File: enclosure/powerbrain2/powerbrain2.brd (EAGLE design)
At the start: 24.8 x 64.8 mm, 45 parts, among them Q2 200mA/50V, Q3 200mA/50V, X2 ZX62D-B-5PA8

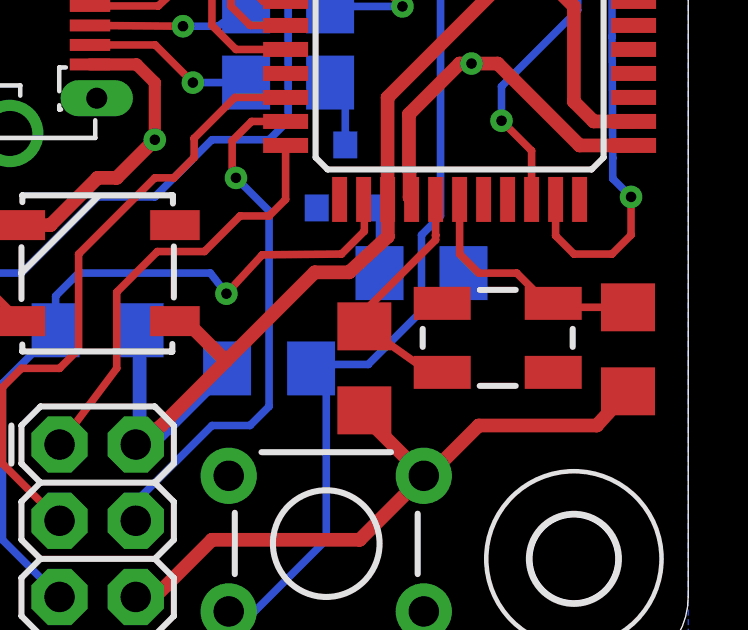
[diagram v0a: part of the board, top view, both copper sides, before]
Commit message: powerbrain
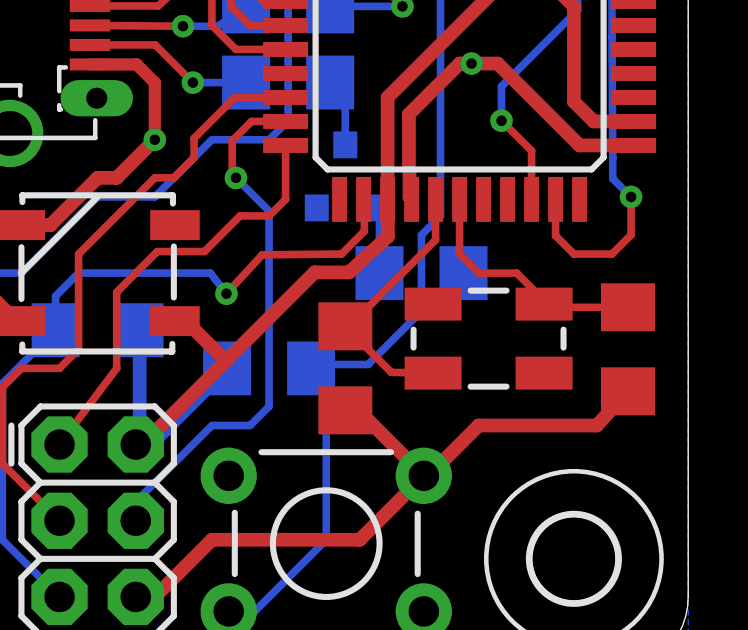
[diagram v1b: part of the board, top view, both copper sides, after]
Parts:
- moved C5 0.63 mm to (13.3, 10.2)
- moved Y1 0.31 mm to (18.1, 11.2)
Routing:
- net N$9: track 8.33 -> 9.08 mm
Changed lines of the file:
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@@
 <setting verticaltext="up"/>
 </settings>
-<grid distance="0.025" unitdist="inch" unit="inch" style="lines" multiple="1" display="yes" altdistance="0.001" altunitdist="inch" altunit="inch"/>
+<grid distance="0.025" unitdist="inch" unit="inch" style="dots" multiple="1" display="yes" altdistance="0.001" altunitdist="inch" altunit="inch"/>
 <layers>
 <layer number="1" name="Top" color="4" fill="1" visible="yes" active="yes"/>
@@
 </element>
 <element name="C4" library="SparkFun-Passives" package="1206" value="22pF" x="22.7584" y="10.795" smashed="yes" rot="R90"/>
-<element name="C5" library="SparkFun-Passives" package="1206" value="22pF" x="13.97" y="10.16" smashed="yes" rot="R90"/>
+<element name="C5" library="SparkFun-Passives" package="1206" value="22pF" x="13.335" y="10.16" smashed="yes" rot="R90"/>
 <element name="C3" library="SparkFun-Passives" package="1206" value="10uF" x="8.89" y="27.305" smashed="yes"/>
-<element name="Y1" library="SparkFun-FreqCtrl" package="CRYSTAL-SMD-5X3" value="" x="18.415" y="11.176" smashed="yes">
-<attribute name="PROD_ID" value="XTAL-08218" x="18.415" y="11.176" size="1.778" layer="27" display="off"/>
-<attribute name="VALUE" x="13.335" y="7.239" size="1.27" layer="27" ratio="10"/>
+<element name="Y1" library="SparkFun-FreqCtrl" package="CRYSTAL-SMD-5X3" value="" x="18.1102" y="11.1506" smashed="yes">
+<attribute name="PROD_ID" value="XTAL-08218" x="18.1102" y="11.1506" size="1.778" layer="27" display="off"/>
+<attribute name="VALUE" x="13.0302" y="7.2136" size="1.27" layer="27" ratio="10"/>
 </element>
 <element name="X2" library="zx62d-b-5pa8-oshpark_10" package="ZX62D-B-5PA8" value="ZX62D-B-5PA8" x="0" y="21.59" smashed="yes">
@@
 <wire x1="10.29" y1="27.305" x2="10.16" y2="27.175" width="0.254" layer="1"/>
 <via x="6.985" y="17.78" extent="1-16" drill="0.35"/>
-<wire x1="13.97" y1="8.76" x2="13.97" y2="8.4328" width="0.254" layer="1"/>
+<wire x1="13.335" y1="8.76" x2="13.97" y2="8.4328" width="0.254" layer="1"/>
 <wire x1="2.503" y1="15.203" x2="2.503" y2="14.935" width="0.254" layer="1"/>
 <wire x1="4.825" y1="20.29" x2="6.38" y2="20.29" width="0.4064" layer="1"/>
@@
 <contactref element="C4" pad="2"/>
 <contactref element="Y1" pad="3"/>
-<wire x1="20.059" y1="12.326" x2="20.265" y2="12.326" width="0.254" layer="1"/>
+<wire x1="20.059" y1="12.326" x2="19.9602" y2="12.3006" width="0.254" layer="1"/>
 <wire x1="20.059" y1="12.326" x2="19.05" y2="13.335" width="0.254" layer="1"/>
 <wire x1="19.05" y1="13.335" x2="17.78" y2="13.335" width="0.254" layer="1"/>
 <wire x1="17.78" y1="13.335" x2="17.145" y2="13.97" width="0.254" layer="1"/>
 <wire x1="17.145" y1="13.97" x2="17.145" y2="15.79" width="0.254" layer="1"/>
-<wire x1="20.265" y1="12.326" x2="20.396" y2="12.195" width="0.254" layer="1"/>
+<wire x1="19.9602" y1="12.3006" x2="20.396" y2="12.195" width="0.254" layer="1"/>
 <wire x1="20.396" y1="12.195" x2="22.7584" y2="12.195" width="0.254" layer="1"/>
 </signal>
@@
 <contactref element="C5" pad="2"/>
 <contactref element="Y1" pad="1"/>
-<wire x1="16.345" y1="14.57" x2="16.345" y2="14.605" width="0.254" layer="1"/>
-<wire x1="16.345" y1="14.605" x2="16.345" y2="15.79" width="0.254" layer="1"/>
-<wire x1="16.565" y1="10.026" x2="16.139" y2="10.026" width="0.254" layer="1"/>
-<wire x1="13.97" y1="11.56" x2="16.139" y2="10.026" width="0.254" layer="1"/>
-<wire x1="16.345" y1="14.605" x2="16.345" y2="14.44" width="0.254" layer="1"/>
+<wire x1="16.345" y1="14.44" x2="16.345" y2="15.79" width="0.254" layer="1"/>
+<wire x1="16.2602" y1="10.0006" x2="14.869" y2="10.026" width="0.254" layer="1"/>
+<wire x1="13.335" y1="11.56" x2="14.869" y2="10.026" width="0.254" layer="1"/>
 <wire x1="16.345" y1="14.44" x2="13.97" y2="12.065" width="0.254" layer="1"/>
-<wire x1="13.97" y1="12.065" x2="13.97" y2="11.56" width="0.254" layer="1"/>
+<wire x1="13.97" y1="12.065" x2="13.335" y2="11.56" width="0.254" layer="1"/>
 </signal>
 <signal name="VBUS_SENSE">
